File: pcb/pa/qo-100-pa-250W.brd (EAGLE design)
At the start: 120 x 60 mm, 1 part

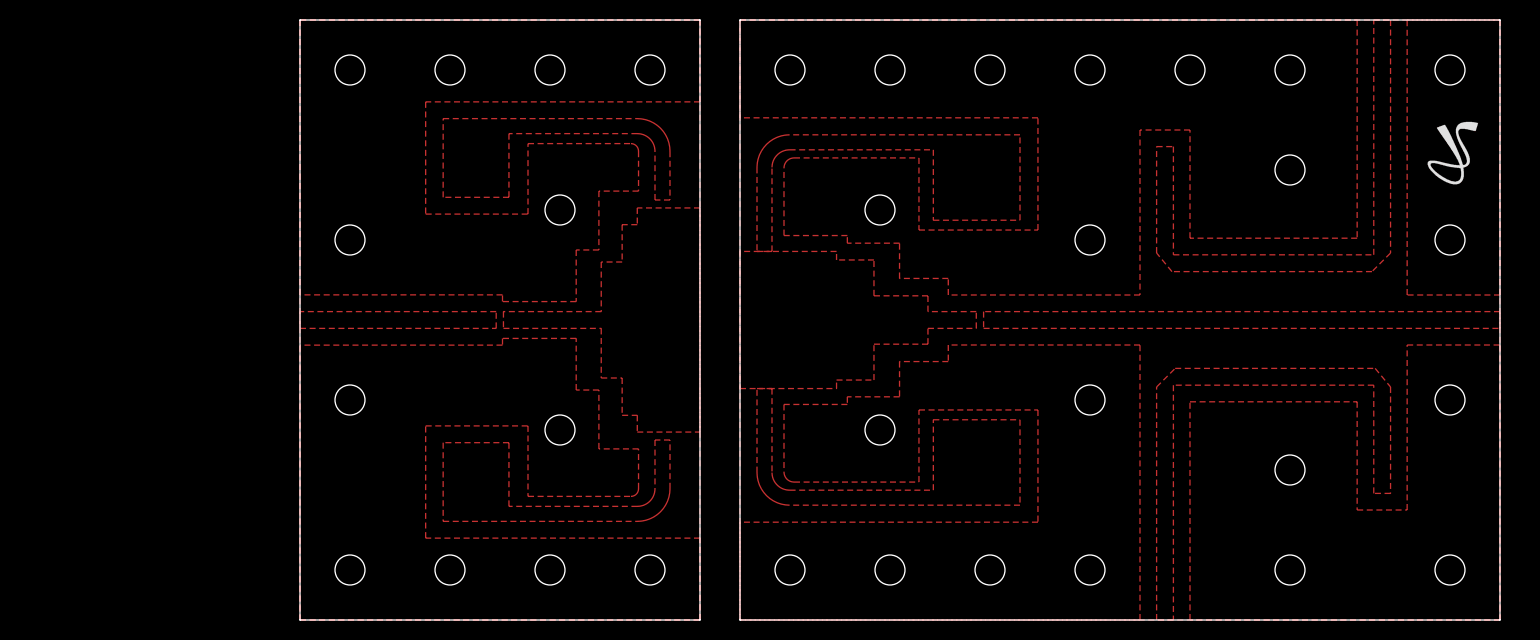
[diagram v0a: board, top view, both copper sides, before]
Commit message: Update PA PCBs
Signed-off-by: João Silva <jgc3silva@gmail.com>
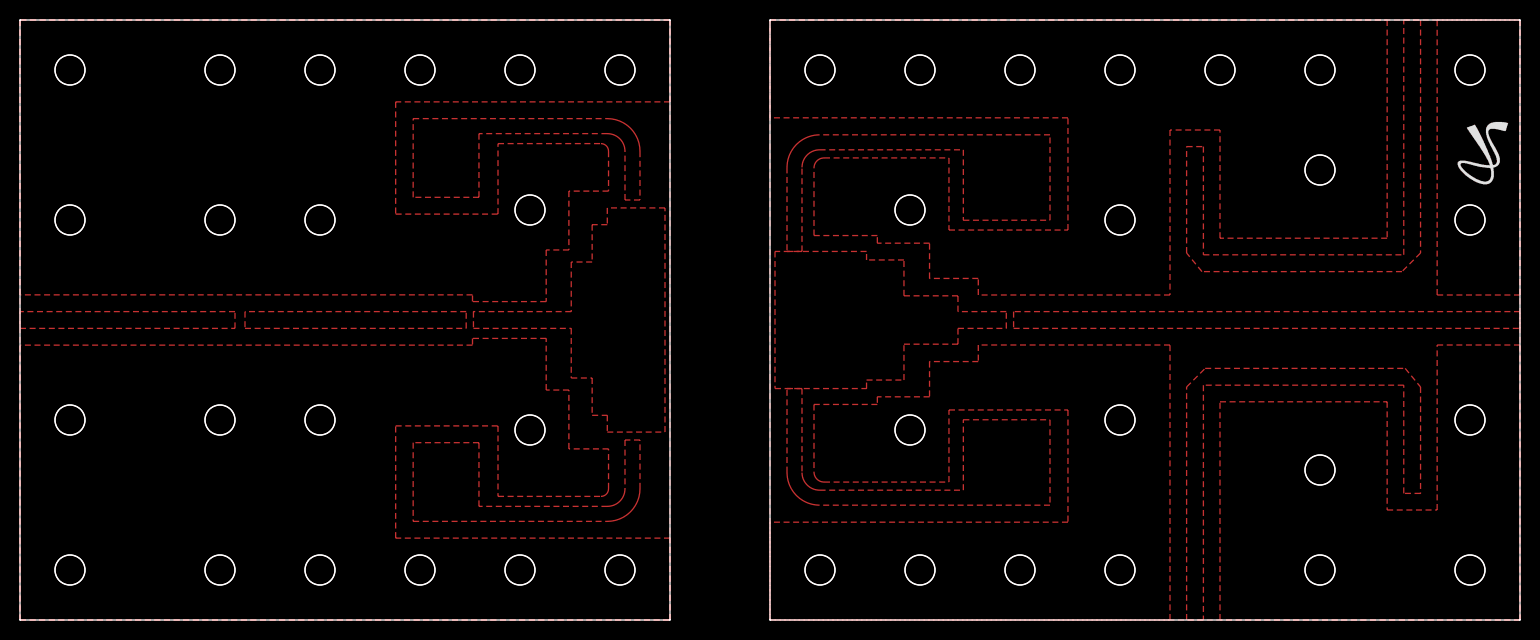
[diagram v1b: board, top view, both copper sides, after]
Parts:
- moved E$1 3.00 mm to (79.0, 50.0)
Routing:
- added copper zone on layer 1, net IN2
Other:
- board size 120 x 60 mm -> 150 x 60 mm
